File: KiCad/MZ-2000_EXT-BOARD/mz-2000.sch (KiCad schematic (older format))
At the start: 5 parts, among them J1 Conn_02x22_Row_Letter_First, J2 Conn_02x22_Row_Letter_First, J4 Jack-DC, J5 Conn_02x22_Row_Letter_First

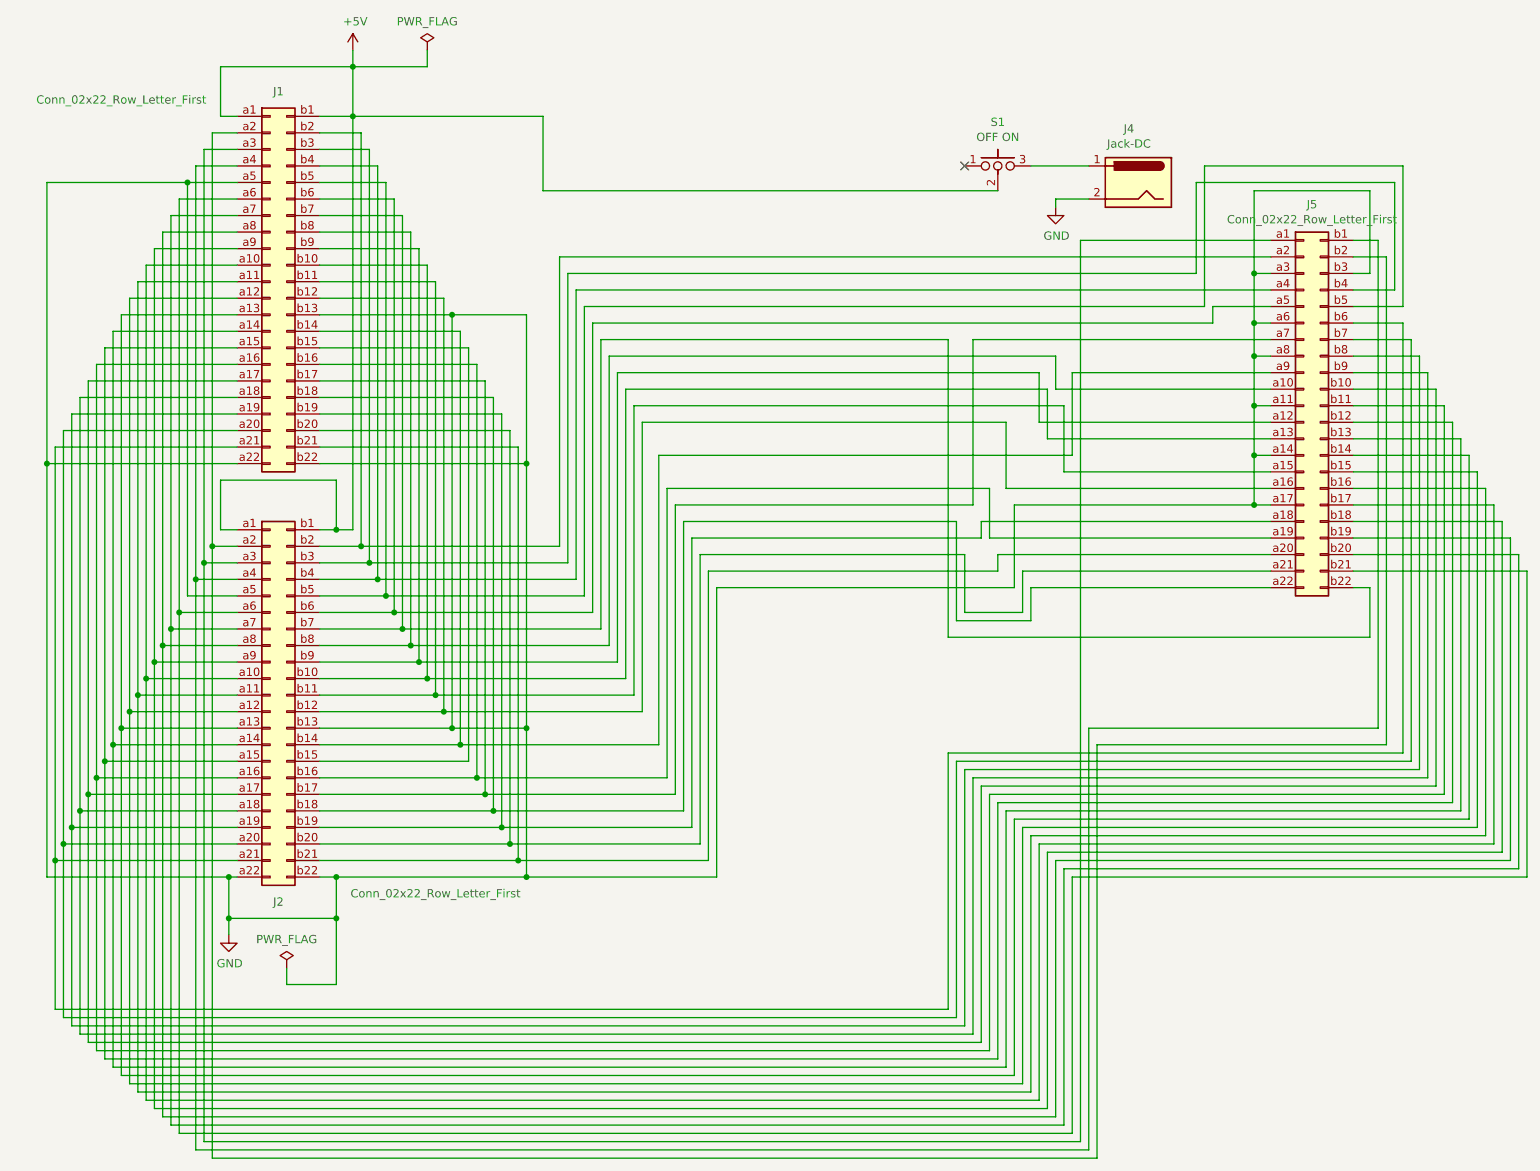
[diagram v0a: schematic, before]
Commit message: Add files via upload
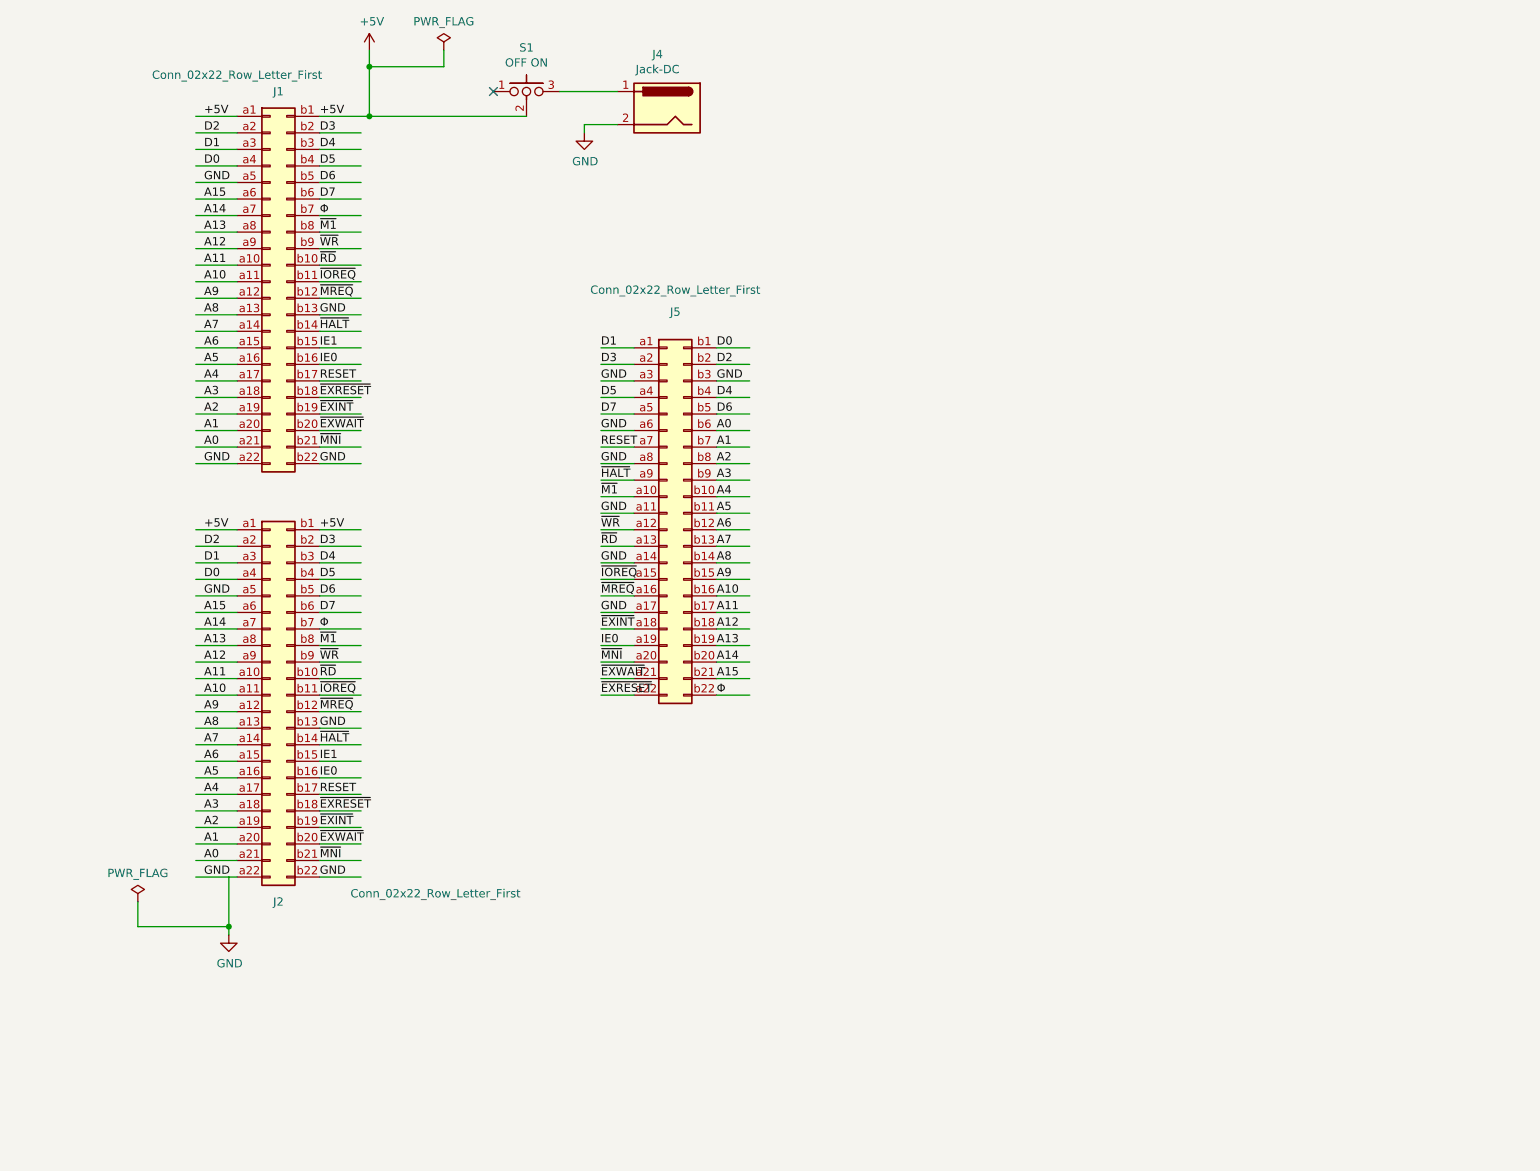
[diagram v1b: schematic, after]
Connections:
- net labels added: A0, A1, A10, A11, A12, A13, A14, A15, A2, A3, A4, A5, A6, A7, A8, A9, D0, D1, D2, D3, D4, D5, D6, D7, IE0, IE1, RESET, ~EXINT, ~EXRESET, ~EXWAIT, ~HALT, ~IOREQ, ~M1, ~MNI, ~MREQ, ~RD, ~WR, Φ
- wire segments 390 -> 144
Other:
- moved on the sheet: J4, J5, S1
